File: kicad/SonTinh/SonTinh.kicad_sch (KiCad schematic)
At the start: 7 parts, among them J1 Screw_Terminal_01x02, J2 Screw_Terminal_01x02, J3 Screw_Terminal_01x02, J4 Screw_Terminal_01x03, U1 BME680

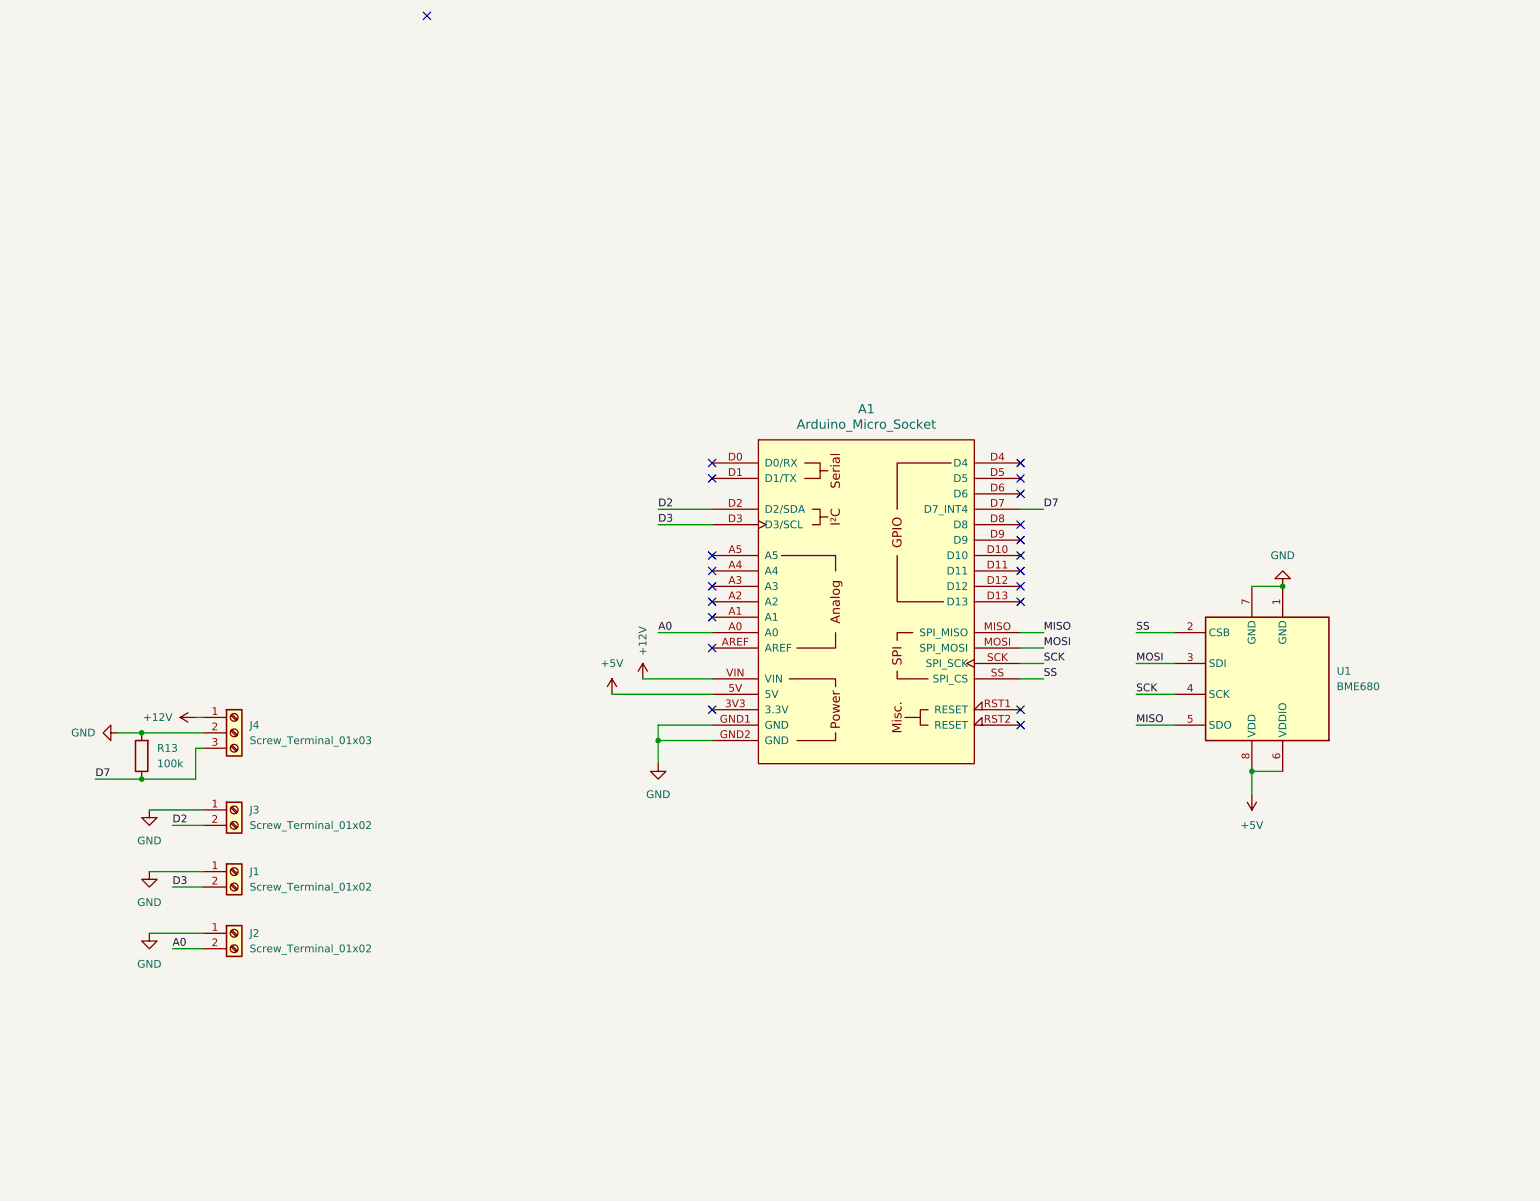
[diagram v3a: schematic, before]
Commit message: The Titans
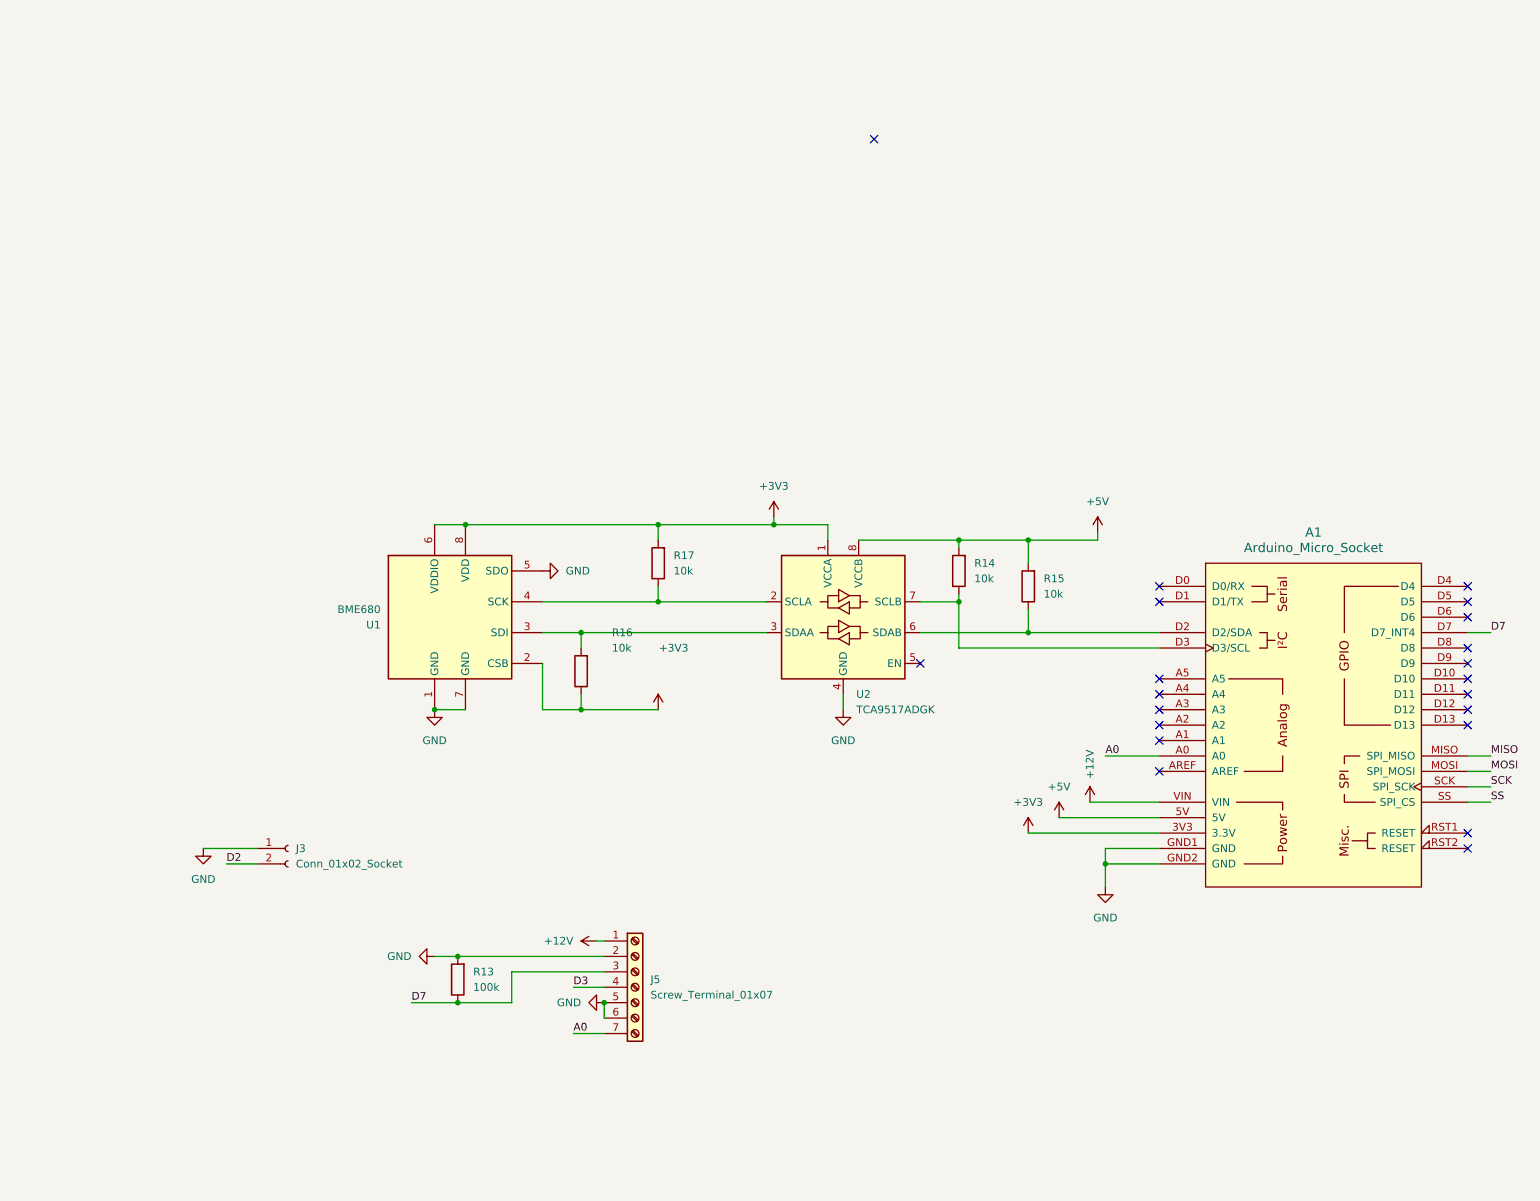
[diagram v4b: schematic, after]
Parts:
- removed J1, J2, J3: Screw_Terminal_01x02, TerminalBlock_Phoenix:TerminalBlock_Phoenix_MPT-0,5-2-2.54_1x02_P2.54mm_Horizontal, symbol Connector:Screw_Terminal_01x02
- removed J4: Screw_Terminal_01x03, TerminalBlock_Phoenix:TerminalBlock_Phoenix_MPT-0,5-3-2.54_1x03_P2.54mm_Horizontal, symbol Connector:Screw_Terminal_01x03
- added J3: Conn_01x02_Socket, Connector_Wire:SolderWire-0.5sqmm_1x02_P4.8mm_D0.9mm_OD2.3mm, symbol Connector:Conn_01x02_Socket
- added J5: Screw_Terminal_01x07, TerminalBlock_WAGO:TerminalBlock_WAGO_233-507_2x07_P2.54mm, symbol Connector:Screw_Terminal_01x07
- added R14, R15, R16, R17: 10k, Resistor_THT:R_Axial_DIN0204_L3.6mm_D1.6mm_P7.62mm_Horizontal, symbol Device:R
- added U2: TCA9517ADGK, Package_SO:VSSOP-8_3x3mm_P0.65mm, symbol Logic_LevelTranslator:TCA9517ADGK
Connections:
- net +12V: now also J5.1 (Pin_1)
- net +5V: now also R14.2, R15.2, U2.8 (VCCB); no longer U1.6 (VDDIO), U1.8 (VDD)
- net A0: now also J5.7 (Pin_7)
- net D2: now also J3.2 (Pin_2); no longer A1.D2 (D2/SDA)
- net D3: now also J5.4 (Pin_4); no longer A1.D3 (D3/SCL)
- net D7: now also J5.3 (Pin_3)
- net GND: now also U1.5 (SDO), J3.1 (Pin_1), J5.2 (Pin_2), J5.5 (Pin_5), J5.6 (Pin_6), U2.4 (GND)
- net MISO: no longer U1.5 (SDO)
- net MOSI: no longer U1.3 (SDI)
- net SCK: no longer U1.4 (SCK)
- net SS: no longer U1.2 (CSB)
- net +3V3: now reaches A1.3V3 (3.3V)
- net +3V3: now also U1.2 (CSB), U1.6 (VDDIO), U1.8 (VDD), R16.1, R17.2, U2.1 (VCCA)
- new net: R17.1, U1.4 (SCK), U2.2 (SCLA)
- new net: R16.2, U1.3 (SDI), U2.3 (SDAA)
- new net: A1.D2 (D2/SDA), R15.1, U2.6 (SDAB)
- new net: A1.D3 (D3/SCL), R14.1, U2.7 (SCLB)
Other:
- moved on the sheet: A1, R13, U1

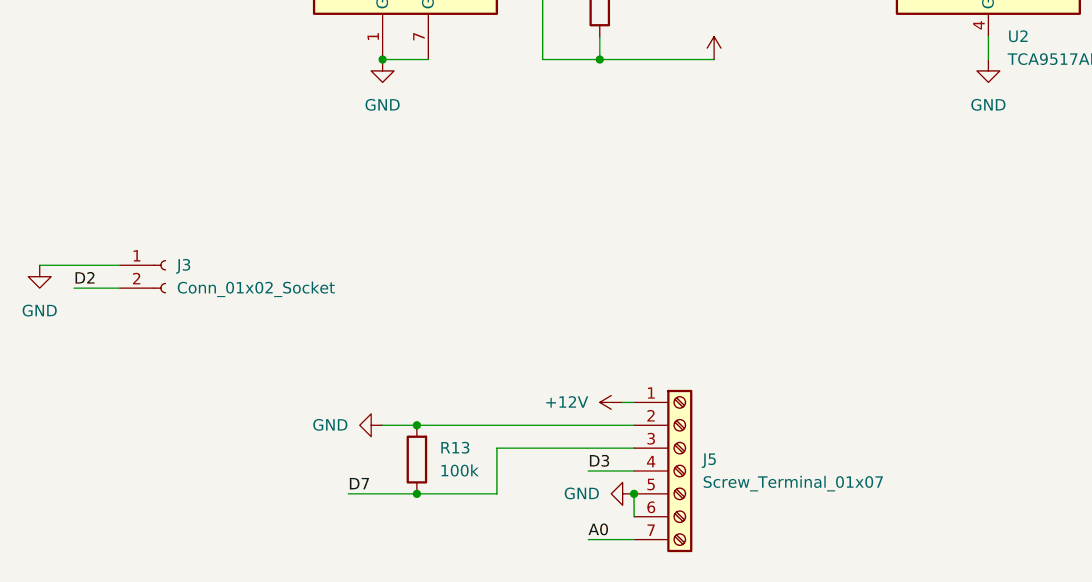
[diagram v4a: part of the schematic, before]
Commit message: Beware Greeks Bearing Gifts
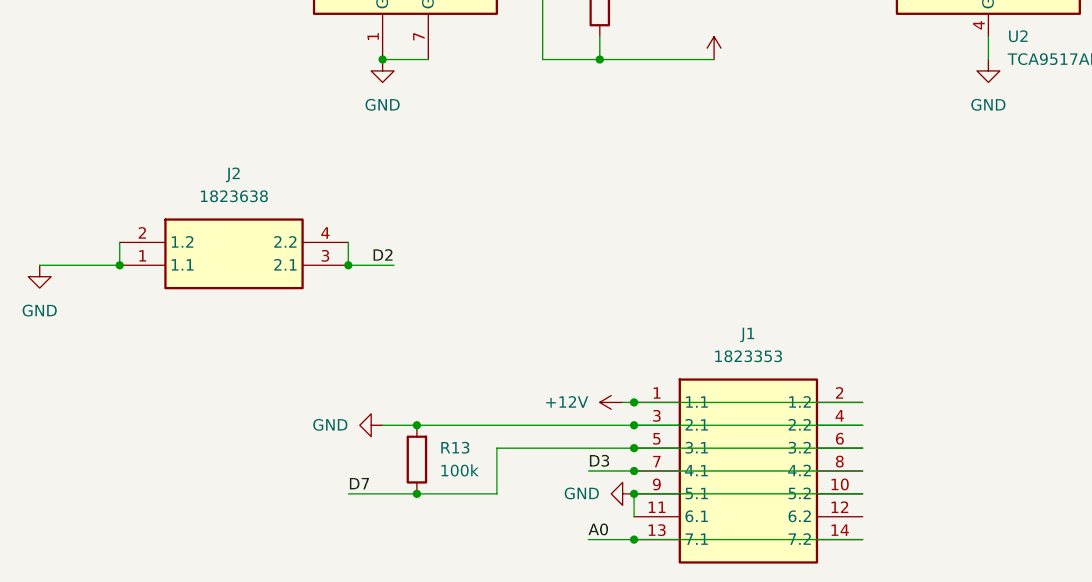
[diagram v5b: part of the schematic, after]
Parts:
- removed J3: Conn_01x02_Socket, Connector_Wire:SolderWire-0.5sqmm_1x02_P4.8mm_D0.9mm_OD2.3mm, symbol Connector:Conn_01x02_Socket
- removed J5: Screw_Terminal_01x07, TerminalBlock_WAGO:TerminalBlock_WAGO_233-507_2x07_P2.54mm, symbol Connector:Screw_Terminal_01x07
- added J1: 1823353, footprints:1823353, symbol PheonixContact:1823353
- added J2: 1823638, footprints:1823638, symbol PheonixContact:1823638
- R13, R14, R15, R16, R17: footprint Resistor_THT:R_Axial_DIN0204_L3.6mm_D1.6mm_P7.62mm_Horizontal -> Resistor_SMD:R_0805_2012Metric
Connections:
- net +12V: now also J1.1 (1.1), J1.2 (1.2)
- net A0: now also J1.13 (7.1), J1.14 (7.2)
- net D2: now also J2.3 (2.1), J2.4 (2.2)
- net D3: now also J1.7 (4.1), J1.8 (4.2)
- net D7: now also J1.5 (3.1), J1.6 (3.2)
- net GND: now also J1.10 (5.2), J1.11 (6.1), J1.3 (2.1), J1.4 (2.2), J1.9 (5.1), J2.1 (1.1), J2.2 (1.2)

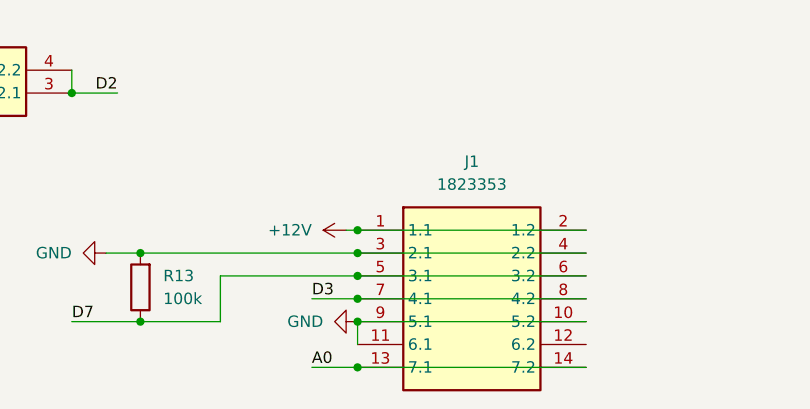
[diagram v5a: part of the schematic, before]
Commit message: Athens City Academy of the Performing Bards
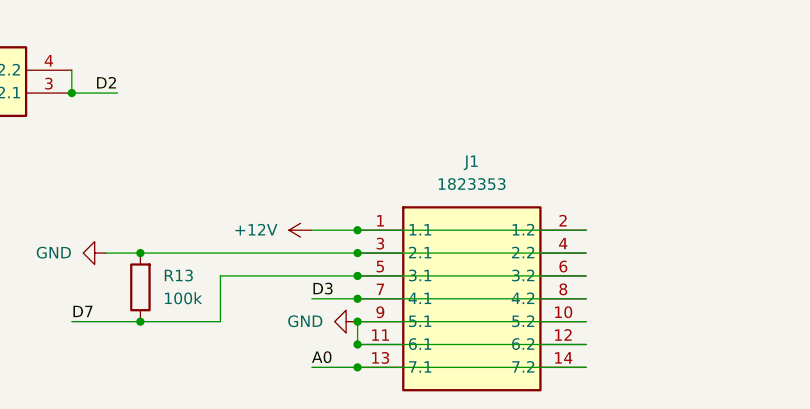
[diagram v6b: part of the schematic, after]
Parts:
- U1: MPN (none) -> BME690
- U2: MPN (none) -> TCA9517ADGKR
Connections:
- net GND: now also J1.12 (6.2)
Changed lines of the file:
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@@
+	)
+	(junction
+		(at 113.03 140.97)
+		(diameter 0)
+		(color 0 0 0 0)
 	)
 	(junction
@@
 	(wire
 		(pts
+			(xy 113.03 140.97) (xy 138.43 140.97)
+		)
+		(stroke
+			(width 0)
+			(type default)
+		)
+	)
+	(wire
+		(pts
 			(xy 259.08 77.47) (xy 255.27 77.47)
 		)
@@
 	(wire
 		(pts
-			(xy 111.76 128.27) (xy 113.03 128.27)
+			(xy 107.95 128.27) (xy 113.03 128.27)
 		)
 		(stroke
@@
 			)
 			(justify left bottom)
+		)
+	)
+	(netclass_flag ""
+		(length 2.54)
+		(shape round)
+		(at 109.22 128.27 0)
+		(fields_autoplaced yes)
+		(effects
+			(font
+				(size 1.27 1.27)
+			)
+			(justify left bottom)
+		)
+		(property "Netclass" "PWR"
+			(at 109.9185 125.73 0)
+			(effects
+				(font
+					(size 1.27 1.27)
+				)
+				(justify left)
+			)
+		)
+		(property "Component Class" ""
+			(at -60.96 19.05 0)
+			(effects
+				(font
+					(size 1.27 1.27)
+					(italic yes)
+				)
+			)
+		)
+	)
+	(netclass_flag ""
+		(length 2.54)
+		(shape round)
+		(at 93.98 130.81 0)
+		(fields_autoplaced yes)
+		(effects
+			(font
+				(size 1.27 1.27)
+			)
+			(justify left bottom)
+		)
+		(property "Netclass" "PWR"
+			(at 94.6785 128.27 0)
+			(effects
+				(font
+					(size 1.27 1.27)
+				)
+				(justify left)
+			)
+		)
+		(property "Component Class" ""
+			(at -76.2 21.59 0)
+			(effects
+				(font
+					(size 1.27 1.27)
+					(italic yes)
+				)
+			)
 		)
 	)
@@
 			)
 		)
+		(property "MPN" "TCA9517ADGKR"
+			(at 152.4 74.93 0)
+			(effects
+				(font
+					(size 1.27 1.27)
+				)
+				(hide yes)
+			)
+		)
 		(pin "5"
 		)
@@
 	(symbol
 		(lib_id "power:+12V")
-		(at 111.76 128.27 90)
+		(at 107.95 128.27 90)
 		(unit 1)
 		(exclude_from_sim no)
@@
 		(dnp no)
 		(property "Reference" "#PWR03"
-			(at 115.57 128.27 0)
+			(at 111.76 128.27 0)
 			(effects
 				(font
@@
 		)
 		(property "Value" "+12V"
-			(at 107.95 128.2699 90)
+			(at 104.14 128.2699 90)
 			(effects
 				(font
@@
 		)
 		(property "Footprint" ""
-			(at 111.76 128.27 0)
+			(at 107.95 128.27 0)
 			(effects
 				(font
@@
 		)
 		(property "Datasheet" ""
-			(at 111.76 128.27 0)
+			(at 107.95 128.27 0)
 			(effects
 				(font
@@
 		)
 		(property "Description" "Power symbol creates a global label with name \"+12V\""
-			(at 111.76 128.27 0)
+			(at 107.95 128.27 0)
 			(effects
 				(font
@@
 			(at 87.63 74.93 0)
 			(effects
+				(font
+					(size 1.27 1.27)
+				)
+				(hide yes)
+			)
+		)
+		(property "MPN" "BME690"
+			(at 87.63 74.93 0)
+			(effects

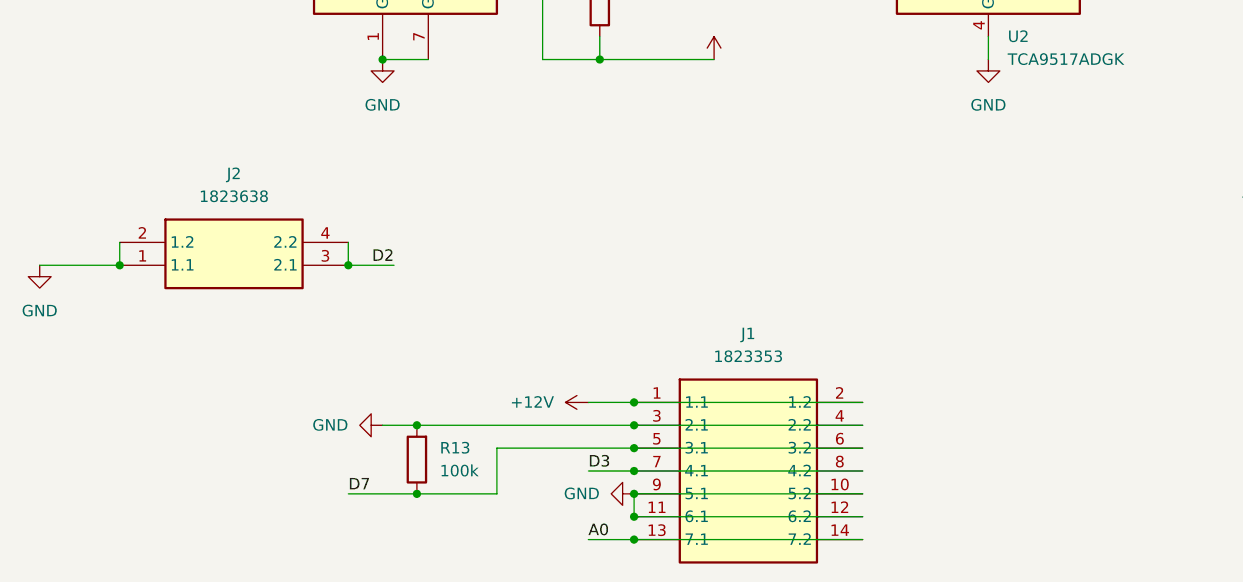
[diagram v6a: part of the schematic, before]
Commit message: A Fistful of Dinars
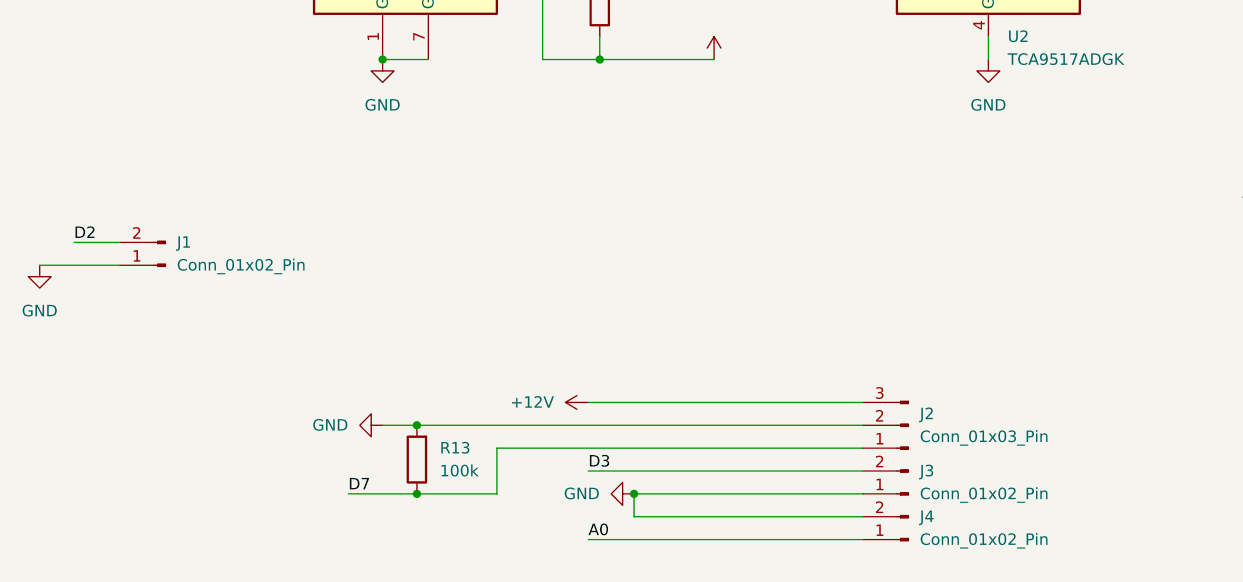
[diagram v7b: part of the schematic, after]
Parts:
- removed J1: 1823353, footprints:1823353, symbol PheonixContact:1823353
- removed J2: 1823638, footprints:1823638, symbol PheonixContact:1823638
- added J1, J3, J4: Conn_01x02_Pin, Connector_Wire:SolderWire-0.75sqmm_1x02_P4.8mm_D1.25mm_OD2.3mm, symbol Connector:Conn_01x02_Pin
- added J2: Conn_01x03_Pin, Connector_Wire:SolderWire-0.75sqmm_1x03_P4.8mm_D1.25mm_OD2.3mm, symbol Connector:Conn_01x03_Pin
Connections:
- net +12V: now also J2.3 (Pin_3)
- net A0: now also J4.1 (Pin_1)
- net D2: now also J1.2 (Pin_2)
- net D3: now also J3.2 (Pin_2)
- net D7: now also J2.1 (Pin_1)
- net GND: now also J1.1 (Pin_1), J2.2 (Pin_2), J3.1 (Pin_1), J4.2 (Pin_2)
